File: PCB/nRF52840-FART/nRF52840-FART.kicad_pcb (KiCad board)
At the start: 2 copper layers, 42.9 x 21.9 mm, 7 parts, among them U1 xiao-ble

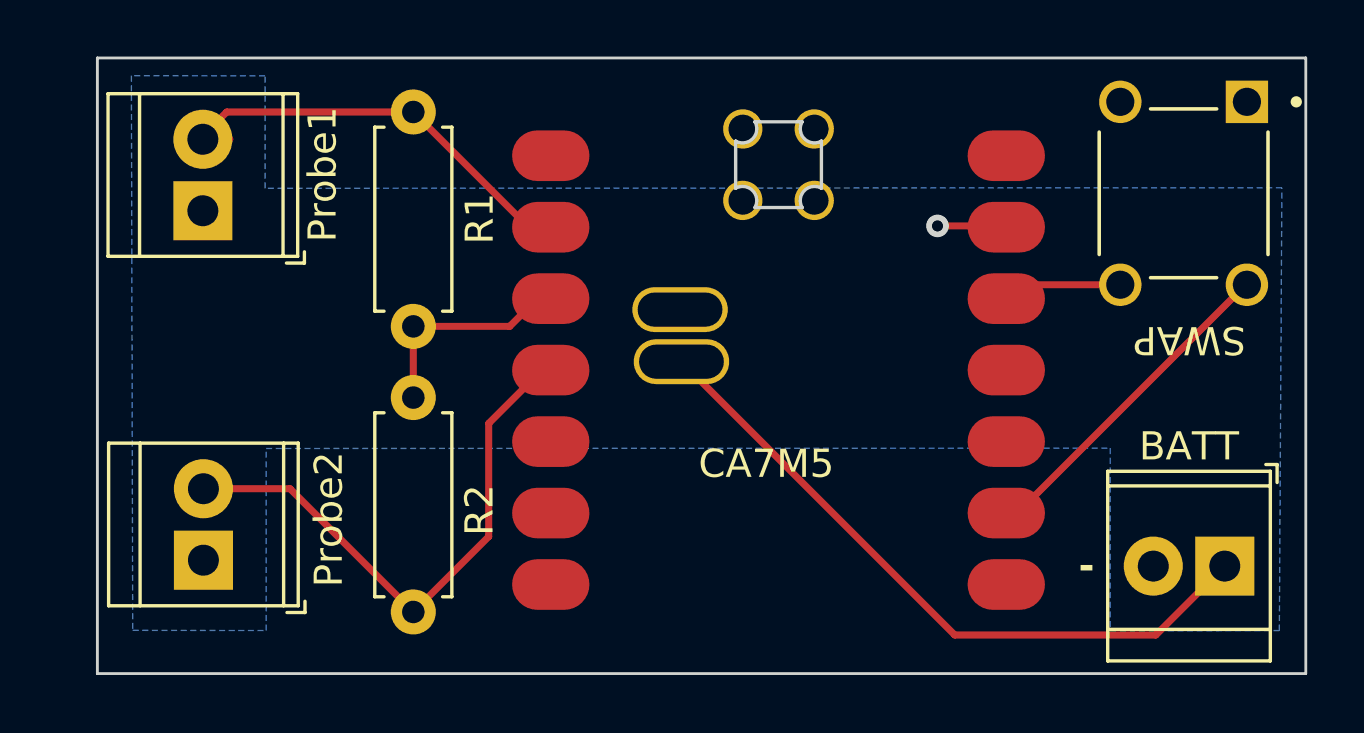
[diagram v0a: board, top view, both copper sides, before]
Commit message: v0.2 of the PCB
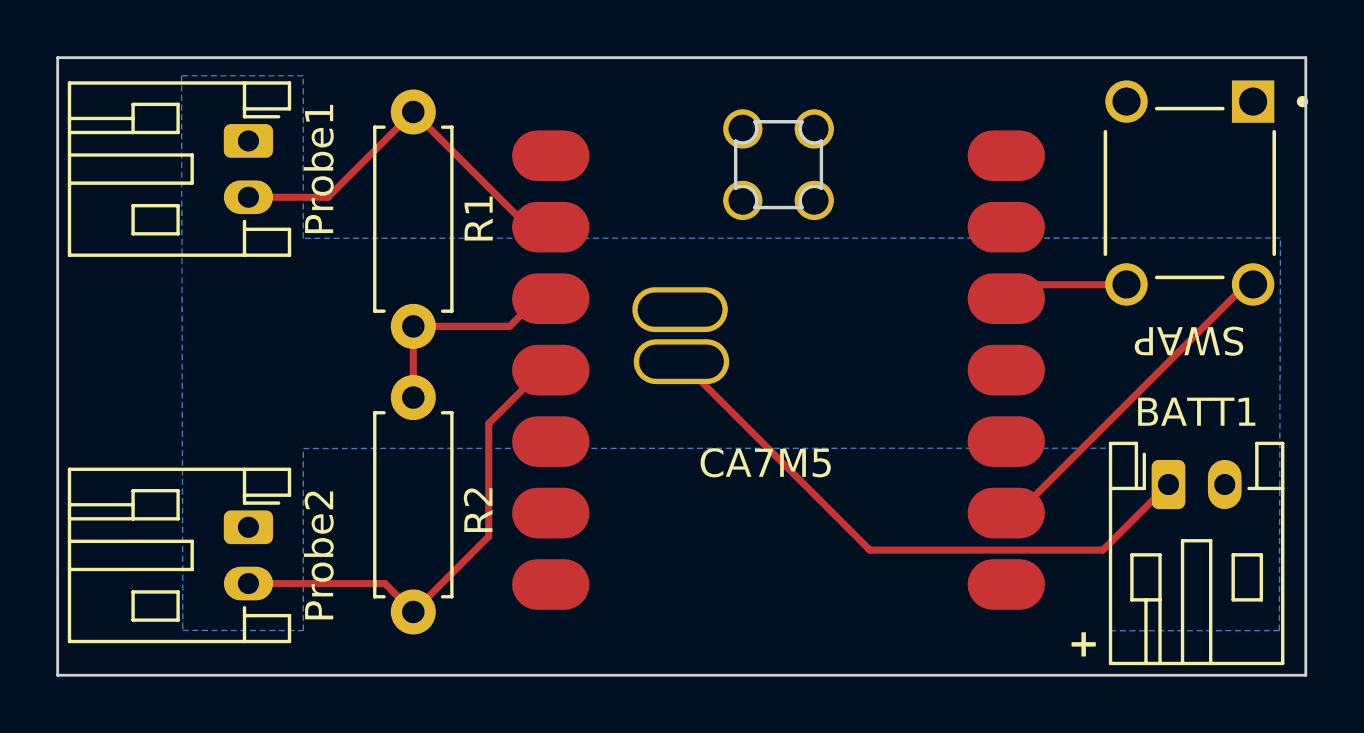
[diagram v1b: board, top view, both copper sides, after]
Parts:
- BATT1: renamed from BATT; footprint TerminalBlock_TE-Connectivity:TerminalBlock_TE_282834-2_1x02_P2.54mm_Horizontal -> Connector_JST:JST_PH_S2B-PH-K_1x02_P2.00mm_Horizontal
- Probe1, Probe2: footprint TerminalBlock_TE-Connectivity:TerminalBlock_TE_282834-2_1x02_P2.54mm_Horizontal -> Connector_JST:JST_PH_S2B-PH-K_1x02_P2.00mm_Horizontal
- moved BATT1 3.52 mm to (93.4, 64.1), turned to 0 degrees
- moved Probe1 2.96 mm to (60.7, 51.9), turned to -90 degrees
- moved Probe2 1.98 mm to (60.7, 65.7), turned to -90 degrees
- moved S1 0.22 mm to (94.1, 53.8)
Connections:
- U1 pad 13: GND -> unconnected-(U1-GND-Pad13)
- U1 pad 15: unconnected-(U1-A30_SWCLK-Pad16) -> unconnected-(U1-A31_SWDIO-Pad15)
- U1 pad 17: unconnected-(U1-A30_SWCLK-Pad16) -> unconnected-(U1-RESET-Pad17)
- U1 pad 18: unconnected-(U1-A30_SWCLK-Pad16) -> unconnected-(U1-GND-Pad18)
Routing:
- net +BATT: track 24.4 -> 21.1 mm
- net /p2reading: track 19.7 -> 16.7 mm
- net GND: track 2.94 -> 0.00 mm, vias 1 -> 0
- net /p1reading: track 15.4 -> 13.6 mm
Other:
- board size 42.9 x 21.9 mm -> 44.4 x 22 mm
- board text added: "+"
- board text removed: "-"
